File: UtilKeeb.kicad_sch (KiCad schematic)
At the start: 126 parts, among them SW1 SW_Push, SW10 SW_Push, SW11 SW_Push, SW12 SW_Push, SW13 SW_Push, SW14 SW_Push, SW15 SW_Push, SW16 SW_Push, SW17 SW_Push, SW18 SW_Push, SW19 SW_Push, SW2 SW_Push, SW20 SW_Push, SW21 SW_Push, SW22 SW_Push, SW23 SW_Push, SW24 SW_Push, SW25 SW_Push, SW26 SW_Push, SW27 SW_Push, SW28 SW_Push, SW29 SW_Push, SW3 SW_Push, SW30 SW_Push, SW31 SW_Push, SW32 SW_Push, SW33 SW_Push, SW34 SW_Push, SW35 SW_Push, SW36 SW_Push, SW37 SW_Push, SW38 SW_Push, SW39 SW_Push, SW4 SW_Push, SW40 SW_Push, SW41 SW_Push, SW42 SW_Push, SW43 SW_Push, SW44 SW_Push, SW45 SW_Push, SW46 SW_Push, SW47 SW_Push, SW48 SW_Push, SW49 SW_Push, SW5 SW_Push, SW50 SW_Push, SW51 SW_Push, SW52 SW_Push, SW53 SW_Push, SW54 SW_Push, SW55 SW_Push, SW56 SW_Push, SW57 SW_Push, SW58 SW_Push, SW59 SW_Push, SW6 SW_Push, SW60 SW_Push, SW61 SW_Push, SW62 SW_Push, SW7 SW_Push, SW8 SW_Push, SW9 SW_Push

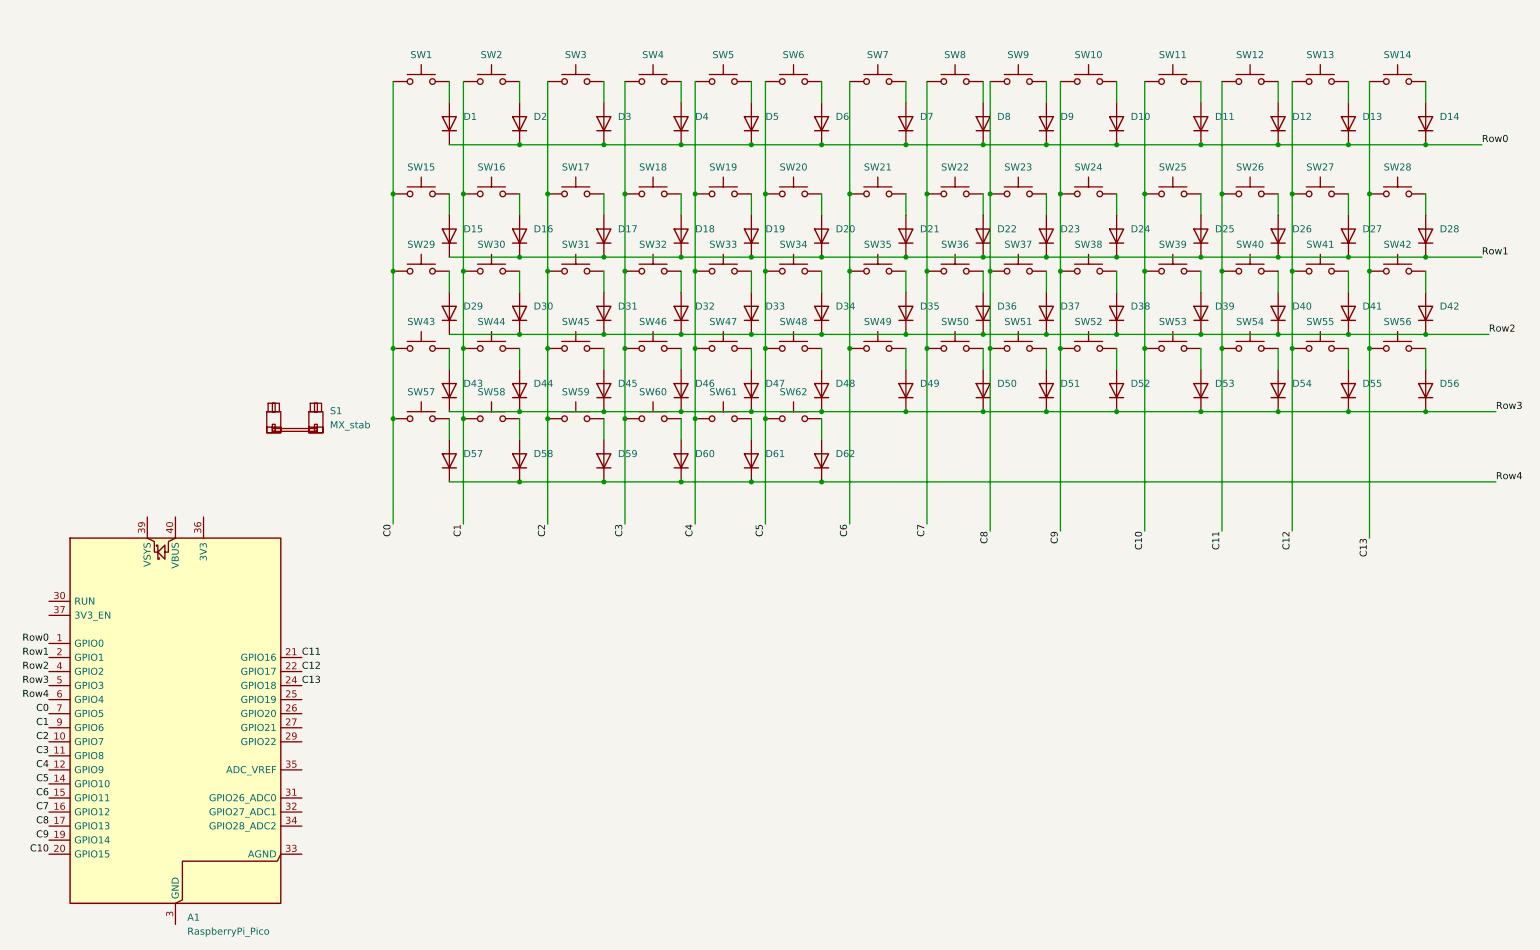
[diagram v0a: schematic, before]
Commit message: Finish for tonight, rebegin tmrw with proper Unit Spacing
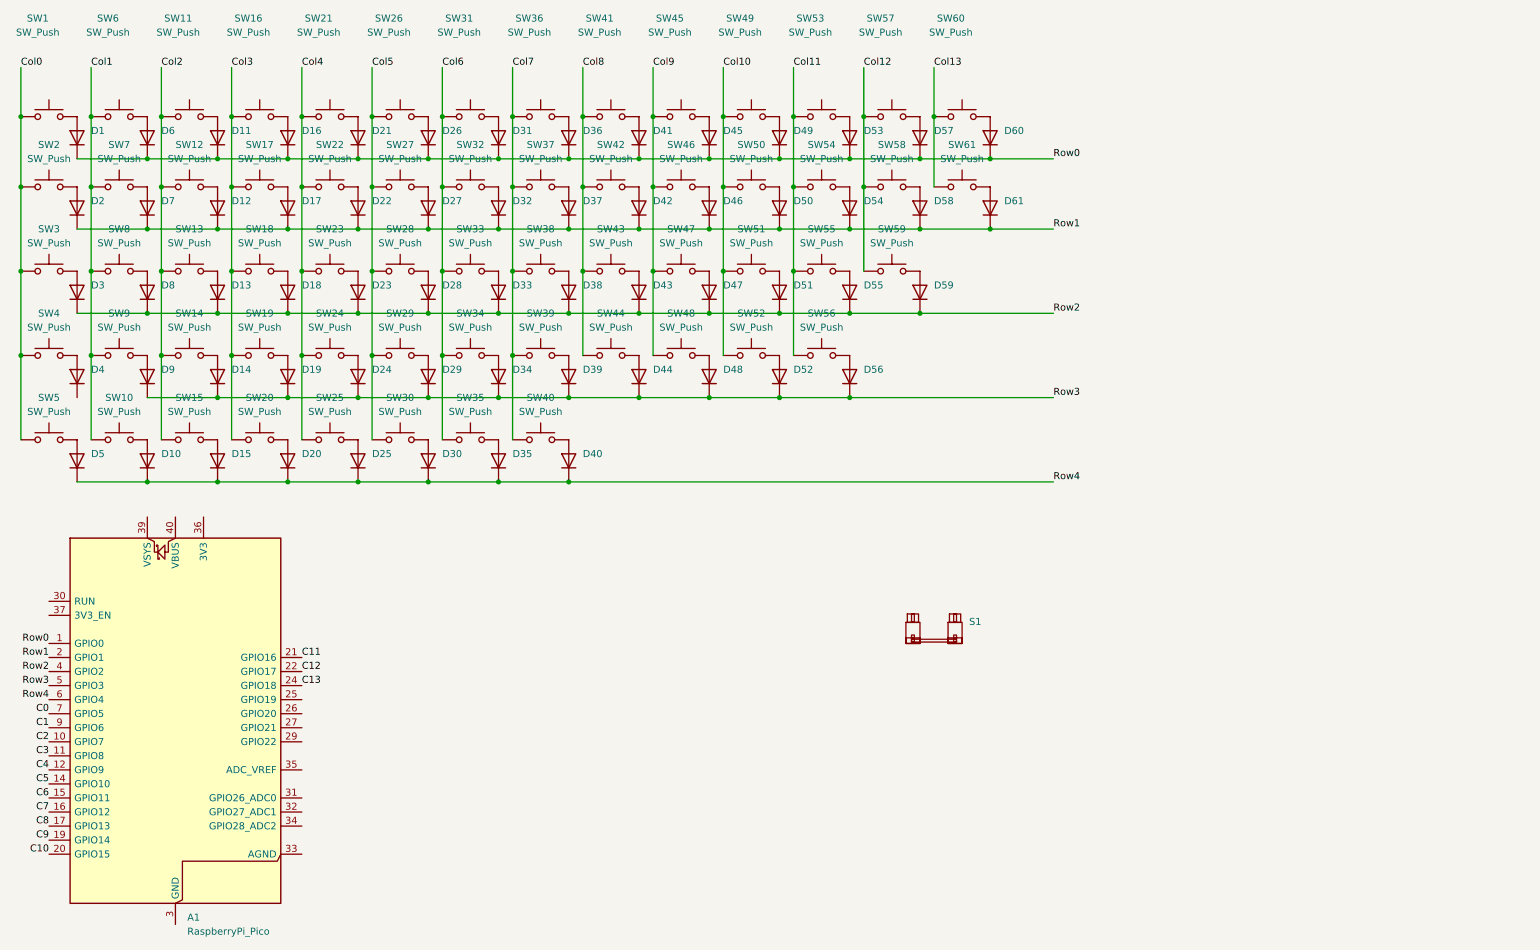
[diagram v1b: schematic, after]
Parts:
- removed D62: 1N4148, Diode_THT:D_DO-35_SOD27_P7.62mm_Horizontal, symbol Diode:1N4148
- removed SW62: SW_Push, PCM_marbastlib-choc:SW_MX_1uWith3DModel, symbol Switch:SW_Push
- SW14, SW42: footprint PCM_marbastlib-mx:SW_MX_1.5u -> PCM_marbastlib-choc:SW_MX_1uWith3DModel
- SW15, SW29: footprint PCM_marbastlib-mx:SW_MX_1.25u -> PCM_marbastlib-choc:SW_MX_1uWith3DModel
- SW2: footprint PCM_marbastlib-choc:SW_MX_1uWith3DModel -> PCM_marbastlib-mx:SW_MX_1.5u
- SW3: footprint PCM_marbastlib-choc:SW_MX_1uWith3DModel -> PCM_marbastlib-mx:SW_MX_1.75u
- SW4: footprint PCM_marbastlib-choc:SW_MX_1uWith3DModel -> PCM_marbastlib-mx:STAB_MX_2.25u
- SW41, SW53: footprint PCM_marbastlib-mx:SW_MX_1.75u -> PCM_marbastlib-choc:SW_MX_1uWith3DModel
- SW5: footprint PCM_marbastlib-choc:SW_MX_1uWith3DModel -> Button_Switch_Keyboard:SW_Cherry_MX_1.25u_PCB
- SW57: footprint marbastlib-mx:SW_MX_1.25u -> PCM_marbastlib-choc:SW_MX_1uWith3DModel
- SW60, SW61: footprint PCM_marbastlib-choc:SW_MX_1uWith3DModel -> PCM_marbastlib-mx:STAB_MX_2u
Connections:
- net C0: no longer SW1.2, SW15.2, SW29.2, SW43.2, SW57.2
- net C1: no longer SW16.2, SW2.2, SW30.2, SW44.2, SW58.2
- net C10: no longer SW11.2, SW25.2, SW39.2, SW53.2
- net C11: no longer SW12.2, SW26.2, SW40.2, SW54.2
- net C12: no longer SW13.2, SW27.2, SW41.2, SW55.2
- net C13: no longer SW14.2, SW28.2, SW42.2, SW56.2
- net C2: no longer SW17.2, SW3.2, SW31.2, SW45.2, SW59.2
- net C3: no longer SW18.2, SW32.2, SW4.2, SW46.2, SW60.2
- net C4: no longer SW19.2, SW33.2, SW47.2, SW5.2, SW61.2
- net C5: no longer SW20.2, SW34.2, SW48.2, SW6.2
- net C6: no longer SW21.2, SW35.2, SW49.2, SW7.2
- net C7: no longer SW22.2, SW36.2, SW50.2, SW8.2
- net C8: no longer SW23.2, SW37.2, SW51.2, SW9.2
- net C9: no longer SW10.2, SW24.2, SW38.2, SW52.2
- net Row0: now also D16.1 (K), D21.1 (K), D26.1 (K), D31.1 (K), D36.1 (K), D41.1 (K), D45.1 (K), D49.1 (K), D53.1 (K), D57.1 (K), D60.1 (K); no longer D10.1 (K), D12.1 (K), D13.1 (K), D14.1 (K), D2.1 (K), D3.1 (K), D4.1 (K), D5.1 (K), D7.1 (K), D8.1 (K), D9.1 (K)
- net Row1: now also D12.1 (K), D2.1 (K), D32.1 (K), D37.1 (K), D42.1 (K), D46.1 (K), D50.1 (K), D54.1 (K), D58.1 (K), D61.1 (K), D7.1 (K); no longer D15.1 (K), D16.1 (K), D18.1 (K), D19.1 (K), D20.1 (K), D21.1 (K), D23.1 (K), D24.1 (K), D25.1 (K), D26.1 (K), D28.1 (K)
- net Row2: now also D13.1 (K), D18.1 (K), D23.1 (K), D28.1 (K), D3.1 (K), D43.1 (K), D47.1 (K), D51.1 (K), D55.1 (K), D59.1 (K), D8.1 (K); no longer D29.1 (K), D30.1 (K), D31.1 (K), D32.1 (K), D34.1 (K), D35.1 (K), D36.1 (K), D37.1 (K), D39.1 (K), D40.1 (K), D41.1 (K), D42.1 (K)
- net Row3: now also D14.1 (K), D19.1 (K), D24.1 (K), D29.1 (K), D34.1 (K), D39.1 (K), D9.1 (K); no longer D43.1 (K), D45.1 (K), D46.1 (K), D47.1 (K), D49.1 (K), D50.1 (K), D51.1 (K), D53.1 (K), D54.1 (K), D55.1 (K)
- net Row4: now also D10.1 (K), D15.1 (K), D20.1 (K), D25.1 (K), D30.1 (K), D35.1 (K), D40.1 (K), D5.1 (K); no longer D57.1 (K), D58.1 (K), D59.1 (K), D60.1 (K), D61.1 (K)
- net at D11.2 (A): now also SW11.2; no longer SW11.1
- net at D60.2 (A): now also SW60.2; no longer SW60.1
- net at D35.2 (A): now also SW35.2; no longer SW35.1
- net at D50.2 (A): now also SW50.2; no longer SW50.1
- net at D26.2 (A): now also SW26.2; no longer SW26.1
- net at D54.2 (A): now also SW54.2; no longer SW54.1
- net at D4.2 (A): now also SW4.2; no longer SW4.1
- net at D2.2 (A): now also SW2.2; no longer SW2.1
- net at D22.2 (A): now also SW22.2; no longer SW22.1
- net at D21.2 (A): now also SW21.2; no longer SW21.1
- net at D30.2 (A): now also SW30.2; no longer SW30.1
- net at D36.2 (A): now also SW36.2; no longer SW36.1
- net at D33.2 (A): now also SW33.2; no longer SW33.1
- net at D17.2 (A): now also SW17.2; no longer SW17.1
- net at D48.2 (A): now also SW48.2; no longer SW48.1
- net at D42.2 (A): now also SW42.2; no longer SW42.1
- net at D29.2 (A): now also SW29.2; no longer SW29.1
- net at D39.2 (A): now also SW39.2; no longer SW39.1
- net at D56.2 (A): now also SW56.2; no longer SW56.1
- net at D20.2 (A): now also SW20.2; no longer SW20.1
- net at D45.2 (A): now also SW45.2; no longer SW45.1
- net at D49.2 (A): now also SW49.2; no longer SW49.1
- net at D10.2 (A): now also SW10.2; no longer SW10.1
- net at D9.2 (A): now also SW9.2; no longer SW9.1
- net at D55.2 (A): now also SW55.2; no longer SW55.1
- net at D25.2 (A): now also SW25.2; no longer SW25.1
- net at D53.2 (A): now also SW53.2; no longer SW53.1
- net at D13.2 (A): now also SW13.2; no longer SW13.1
- net at D41.2 (A): now also SW41.2; no longer SW41.1
- net at D27.2 (A): now also SW27.2; no longer SW27.1
- net at D51.2 (A): now also SW51.2; no longer SW51.1
- net at D7.2 (A): now also SW7.2; no longer SW7.1
- net at D23.2 (A): now also SW23.2; no longer SW23.1
- net at D52.2 (A): now also SW52.2; no longer SW52.1
- net at D8.2 (A): now also SW8.2; no longer SW8.1
- net at D46.2 (A): now also SW46.2; no longer SW46.1
- net at D16.2 (A): now also SW16.2; no longer SW16.1
- net at D24.2 (A): now also SW24.2; no longer SW24.1
- net at D32.2 (A): now also SW32.2; no longer SW32.1
- net at D40.2 (A): now also SW40.2; no longer SW40.1
- net at D44.2 (A): now also SW44.2; no longer SW44.1
- net at D1.2 (A): now also SW1.2; no longer SW1.1
- net at D6.2 (A): now also SW6.2; no longer SW6.1
- net at D34.2 (A): now also SW34.2; no longer SW34.1
- net at D37.2 (A): now also SW37.2; no longer SW37.1
- net at D31.2 (A): now also SW31.2; no longer SW31.1
- net at D12.2 (A): now also SW12.2; no longer SW12.1
- net at D57.2 (A): now also SW57.2; no longer SW57.1
- net at D19.2 (A): now also SW19.2; no longer SW19.1
- net at D5.2 (A): now also SW5.2; no longer SW5.1
- net at D14.2 (A): now also SW14.2; no longer SW14.1
- net at D47.2 (A): now also SW47.2; no longer SW47.1
- net at D38.2 (A): now also SW38.2; no longer SW38.1
- net at D18.2 (A): now also SW18.2; no longer SW18.1
- net at D28.2 (A): now also SW28.2; no longer SW28.1
- net at D43.2 (A): now also SW43.2; no longer SW43.1
- net at D59.2 (A): now also SW59.2; no longer SW59.1
- net at D3.2 (A): now also SW3.2; no longer SW3.1
- net at D15.2 (A): now also SW15.2; no longer SW15.1
- net at D61.2 (A): now also SW61.2; no longer SW61.1
- net at D58.2 (A): now also SW58.2; no longer SW58.1
- new net Col0: SW1.1, SW2.1, SW3.1, SW4.1, SW5.1
- new net Col1: SW10.1, SW6.1, SW7.1, SW8.1, SW9.1
- new net Col10: SW49.1, SW50.1, SW51.1, SW52.1
- new net Col11: SW53.1, SW54.1, SW55.1, SW56.1
- new net Col12: SW57.1, SW58.1, SW59.1
- new net Col13: SW60.1, SW61.1
- new net Col2: SW11.1, SW12.1, SW13.1, SW14.1, SW15.1
- new net Col3: SW16.1, SW17.1, SW18.1, SW19.1, SW20.1
- new net Col4: SW21.1, SW22.1, SW23.1, SW24.1, SW25.1
- new net Col5: SW26.1, SW27.1, SW28.1, SW29.1, SW30.1
- new net Col6: SW31.1, SW32.1, SW33.1, SW34.1, SW35.1
- new net Col7: SW36.1, SW37.1, SW38.1, SW39.1, SW40.1
- new net Col8: SW41.1, SW42.1, SW43.1, SW44.1
- new net Col9: SW45.1, SW46.1, SW47.1, SW48.1
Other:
- moved on the sheet: S1
